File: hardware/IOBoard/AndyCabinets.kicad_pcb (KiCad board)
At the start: 2 copper layers, 44.5 x 76.2 mm, 47 parts, among them SW1 Mode_Encoder, SW2 Color_Encoder, U1 74HC14

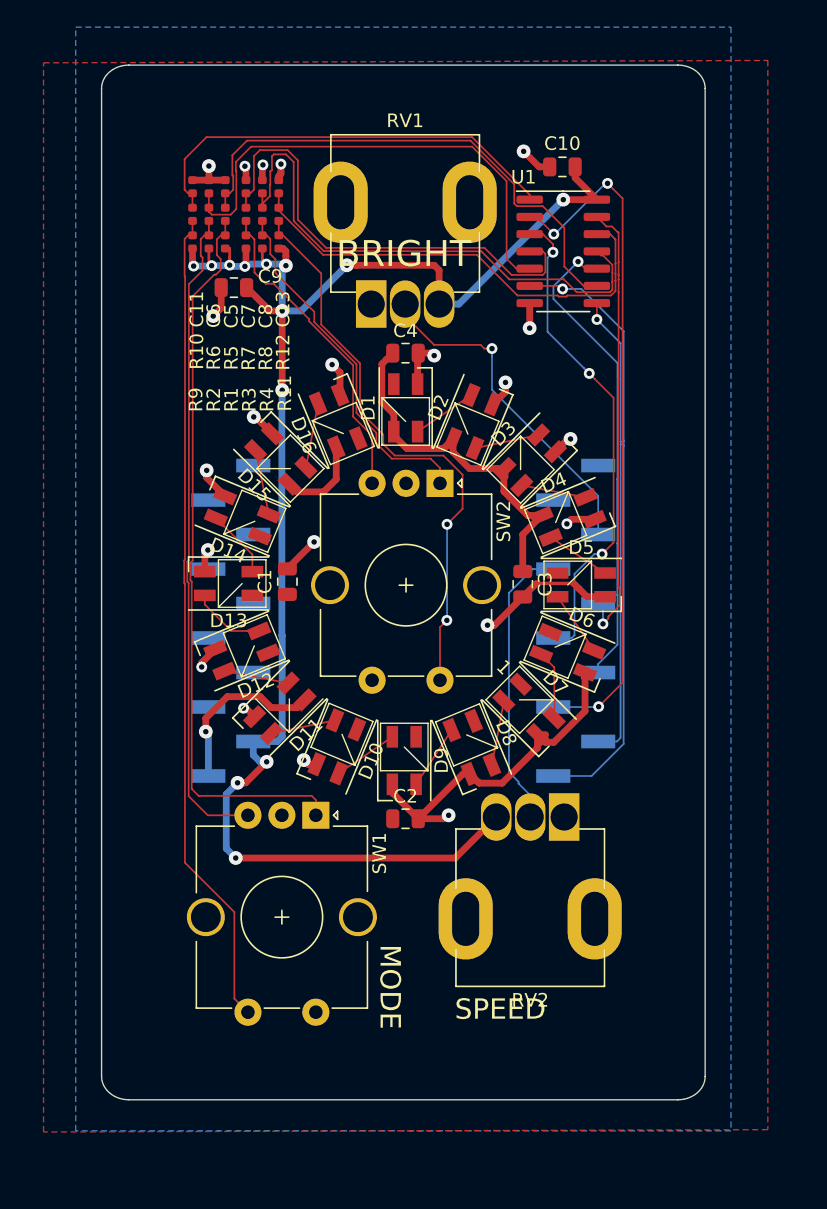
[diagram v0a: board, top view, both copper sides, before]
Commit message: After PCB v2
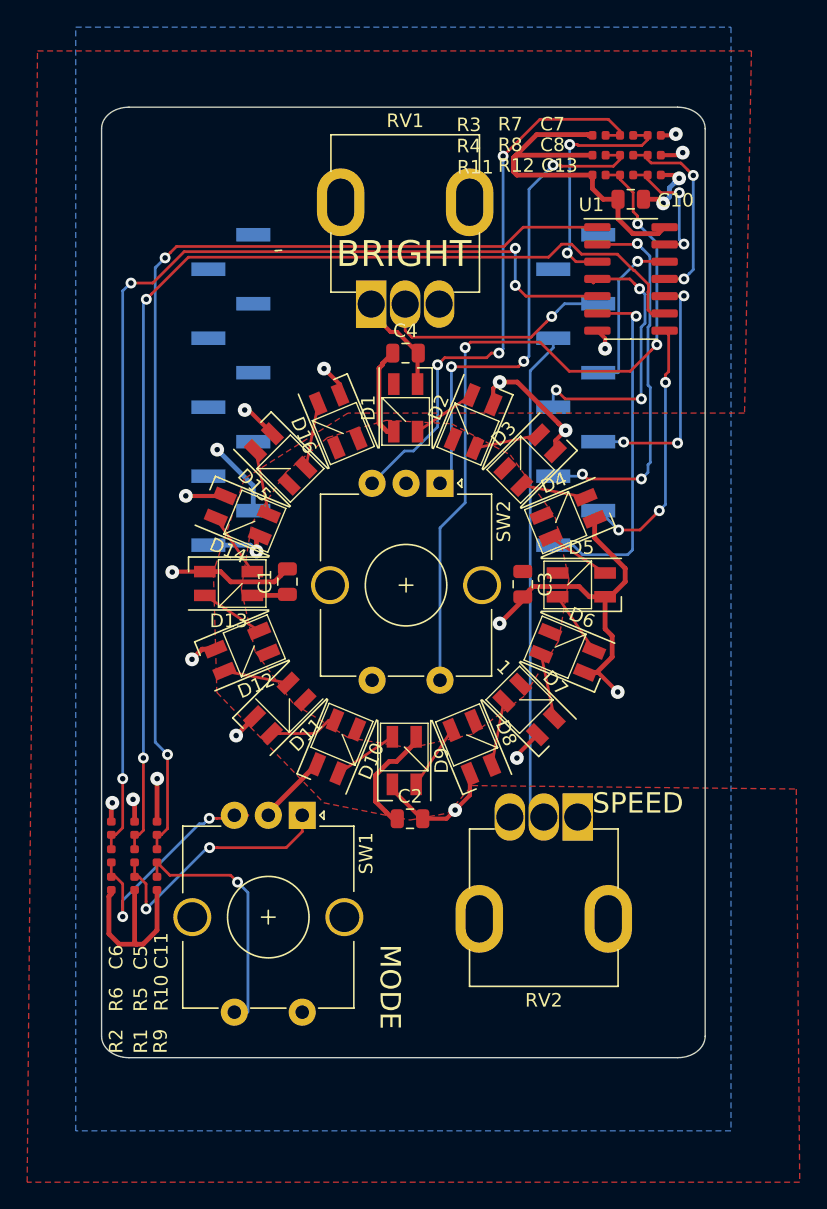
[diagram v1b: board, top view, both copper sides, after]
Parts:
- removed C9: 1uF, Capacitor_SMD:C_0805_2012Metric
- C11, C13: value 0.01uF -> 0.1uF
- moved C6 47.8 mm to (176.1, 115.9)
- moved R2 47.8 mm to (176.1, 120.0)
- moved R6 47.8 mm to (176.1, 117.9)
- moved C5 47.7 mm to (177.8, 115.9)
- moved R1 47.7 mm to (177.8, 120.0)
- moved R5 47.7 mm to (177.8, 117.9)
- moved C11 47.3 mm to (179.5, 115.9)
- moved R10 47.3 mm to (179.5, 117.9)
- moved R9 47.3 mm to (179.5, 120.0)
- moved C7 30.3 mm to (216.1, 64.9), turned to 0 degrees
- moved C8 29.0 mm to (216.1, 66.4), turned to 0 degrees
- moved R7 28.6 mm to (214.1, 64.9), turned to 0 degrees
- moved C13 27.7 mm to (216.1, 67.8), turned to 0 degrees
- moved R8 27.2 mm to (214.1, 66.4), turned to 180 degrees
- moved R3 27.2 mm to (212.0, 64.9), turned to 0 degrees
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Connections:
- U1 pad 12: Net-(C13-Pad1) -> /GPIO32_MODE_BTN
- U1 pad 13: /GPIO32_MODE_BTN -> Net-(C13-Pad1)
- U1 pad 3: /GPIO33_MODE_B -> Net-(C7-Pad1)
- U1 pad 4: Net-(C7-Pad1) -> /GPIO33_MODE_B
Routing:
- net +3V3: track 122.2 -> 48.3 mm, vias 13 -> 1
- net Net-(C5-Pad1): track 38.5 -> 84.1 mm, vias 0 -> 2
- net Net-(C11-Pad1): track 32.2 -> 77.5 mm, vias 0 -> 2
- net Net-(C6-Pad1): track 36.3 -> 81.0 mm, vias 0 -> 4
- net Net-(R10-Pad2): track 60.7 -> 17.5 mm, vias 0 -> 1
- net Net-(R1-Pad2): track 54.0 -> 18.8 mm, vias 0 -> 2
- net Net-(R2-Pad2): track 48.8 -> 17.5 mm, vias 0 -> 2
- net Net-(C8-Pad1): track 40.5 -> 14.6 mm, vias 0 -> 2
- net GNDD: track 74.3 -> 99.1 mm, vias 21 -> 20
- net Net-(C13-Pad1): track 34.2 -> 9.48 mm, vias 0 -> 2
- net +5V: track 46.3 -> 22.6 mm
- net /GPIO35_COLOR_BTN: track 50.9 -> 27.8 mm
- net /GPIO32_MODE_BTN: track 33.1 -> 12.3 mm
- net /GPIO39_COLOR_A: track 44.9 -> 26.5 mm
- net Net-(R3-Pad2): track 24.3 -> 42.1 mm, vias 0 -> 3
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- added copper zone on F.Cu, net +3V3
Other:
- board size 44.5 x 76.2 mm -> 44.4 x 70 mm
- net class Default: clearance 0.1016 -> 0.1524; trace_width 0.127 -> 0.2032
- net class Power: clearance 0.2 -> 0.1524; trace_width 0.5 -> 0.3556
- rule trace_clearance: 0.1016 -> 0.1524
